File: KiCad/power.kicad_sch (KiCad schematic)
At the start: 10 parts

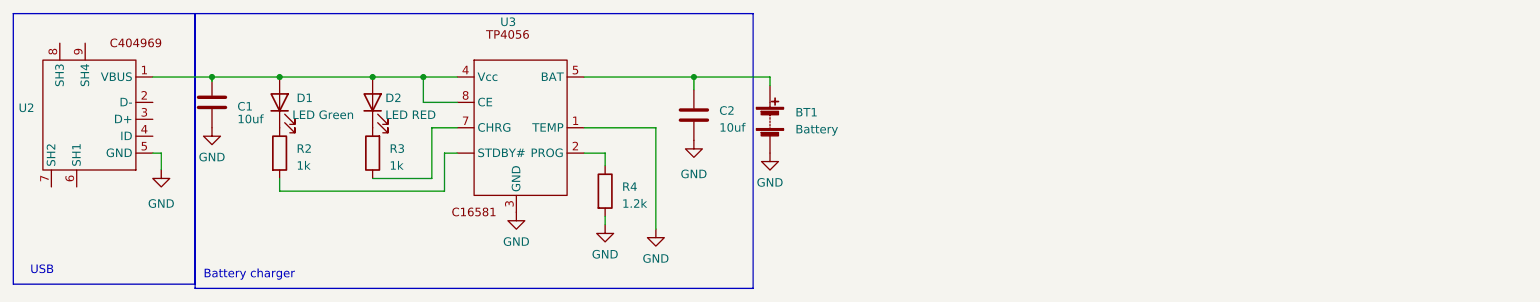
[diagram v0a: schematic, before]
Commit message: kian made som changes to the scmatices
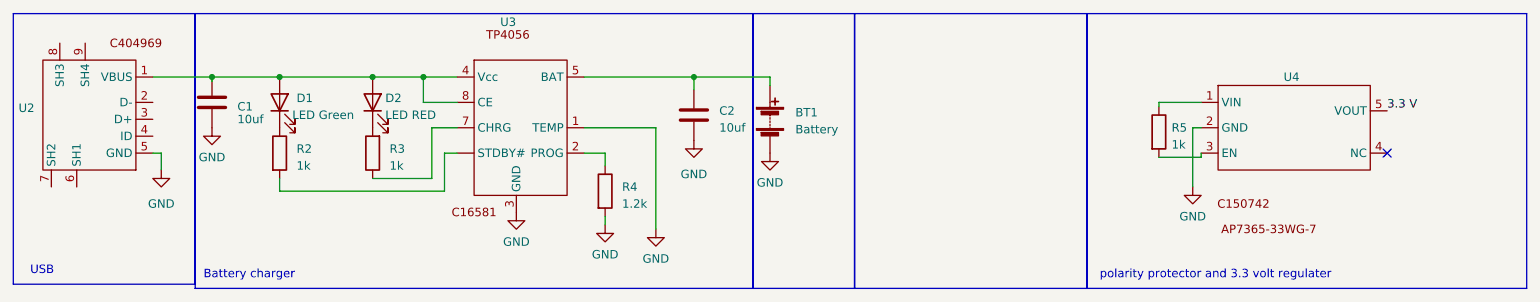
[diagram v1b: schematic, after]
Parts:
- added R5: 1k, symbol Device:R
- added U4: ~, symbol Power comonentes:C150742_(LDO/_UVLO)
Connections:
- net GND: now also U4.2 (GND)
- new net: R5.1, U4.1 (VIN)
- new net: R5.2, U4.3 (EN)
- new net 3.3 V: U4.5 (VOUT)
- no-connect marks 0 -> 1
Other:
- note added: "polarity protector and 3.3 volt regulater"
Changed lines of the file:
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@@
   (junction (at 63.5 30.48) (diameter 0) (color 0 0 0 0)
   )
+  (no_connect (at 229.87 41.91))
   (wire (pts (xy 44.45 41.91) (xy 45.72 41.91))
     (stroke (width 0) (type default))
@@
     (stroke (width 0) (type default))
   )
+  (wire (pts (xy 195.58 34.29) (xy 201.93 34.29))
+    (stroke (width 0) (type default))
+  )
   (wire (pts (xy 53.34 30.48) (xy 63.5 30.48))
     (stroke (width 0) (type default))
   )
+  (wire (pts (xy 195.58 42.545) (xy 201.93 42.545))
+    (stroke (width 0) (type default))
+  )
   (wire (pts (xy 137.16 30.48) (xy 137.16 31.75))
     (stroke (width 0) (type default))
@@
     (stroke (width 0) (type default))
   )
+  (wire (pts (xy 201.93 42.545) (xy 201.93 41.91))
+    (stroke (width 0) (type default))
+  )
   (wire (pts (xy 109.22 30.48) (xy 125.73 30.48))
     (stroke (width 0) (type default))
@@
     (stroke (width 0) (type default))
   )
+  (wire (pts (xy 195.58 34.925) (xy 195.58 34.29))
+    (stroke (width 0) (type default))
+  )
   (wire (pts (xy 85.09 34.29) (xy 85.09 30.48))
     (stroke (width 0) (type default))
@@
     (stroke (width 0) (type default))
   )
+  (wire (pts (xy 200.66 38.1) (xy 201.93 38.1))
+    (stroke (width 0) (type default))
+  )
   (wire (pts (xy 85.09 30.48) (xy 90.17 30.48))
     (stroke (width 0) (type default))
@@
     (stroke (width 0) (type default))
   )
+  (wire (pts (xy 200.66 38.1) (xy 200.66 46.99))
+    (stroke (width 0) (type default))
+  )
   (wire (pts (xy 88.265 41.91) (xy 90.17 41.91))
     (stroke (width 0) (type default))
@@
     (stroke (width 0) (type default))
   )
+  (rectangle (start 134.62 20.955) (end 149.86 62.23)
+    (stroke (width 0) (type default))
+    (fill (type none))
+  )
   (rectangle (start 50.8 20.955) (end 134.62 62.23)
     (stroke (width 0) (type default))
     (fill (type none))
   )
+  (rectangle (start 149.86 20.955) (end 184.785 62.23)
+    (stroke (width 0) (type default))
+    (fill (type none))
+  )
   (rectangle (start 23.495 20.955) (end 50.8 61.595)
+    (stroke (width 0) (type default))
+    (fill (type none))
+  )
+  (rectangle (start 184.785 20.955) (end 250.825 62.23)
     (stroke (width 0) (type default))
     (fill (type none))
@@
   )
   (text "USB" (at 26.035 60.325 0)
+    (effects (font (size 1.27 1.27)) (justify left bottom))
+  )
+  (text "polarity protector and 3.3 volt regulater" (at 186.69 60.96 0)
+    (effects (font (size 1.27 1.27)) (justify left bottom))
+  )
+  (label "3.3 V" (at 229.87 35.56 0) (fields_autoplaced)
     (effects (font (size 1.27 1.27)) (justify left bottom))
   )
@@
         )
       )
+      (project "power"
+        (path "/d9c34bc1-cf5e-42ef-a2b2-2cfbae723006"
+          (reference "D2") (unit 1)
+        )
+      )
       (project "tep work"
         (path "/dbd26d19-6d63-47f2-b172-340d78bc82ae"
@@
         )
       )
-      (project "tep work"
-        (path "/dbd26d19-6d63-47f2-b172-340d78bc82ae"
+      (project "power"
+        (path "/d9c34bc1-cf5e-42ef-a2b2-2cfbae723006"
           (reference "#PWR07") (unit 1)
         )
       )
+      (project "tep work"
+        (path "/dbd26d19-6d63-47f2-b172-340d78bc82ae"
+          (reference "#PWR07") (unit 1)
+        )
+      )
     )
   )
@@
         )
       )
+      (project "power"
+        (path "/d9c34bc1-cf5e-42ef-a2b2-2cfbae723006"
+          (reference "#PWR013") (unit 1)
+        )
+      )
       (project "tep work"
         (path "/dbd26d19-6d63-47f2-b172-340d78bc82ae"
@@
         )
       )
+      (project "power"
+        (path "/d9c34bc1-cf5e-42ef-a2b2-2cfbae723006"
+          (reference "#PWR08") (unit 1)
+        )
+      )
       (project "tep work"
         (path "/dbd26d19-6d63-47f2-b172-340d78bc82ae"
@@
       (project "EEE3088F_CKR"
         (path "/31e5d740-f3fb-4029-be8d-dfdc4f653d72/d53a003e-af2e-46c6-8ee9-c5701cef8adb"
+          (reference "#PWR011") (unit 1)
+        )
+      )
+      (project "power"
+        (path "/d9c34bc1-cf5e-42ef-a2b2-2cfbae723006"
           (reference "#PWR011") (unit 1)
         )
@@
         )
       )
+      (project "power"
+        (path "/d9c34bc1-cf5e-42ef-a2b2-2cfbae723006"
+          (reference "D1") (unit 1)
+        )
+      )
       (project "tep work"
         (path "/dbd26d19-6d63-47f2-b172-340d78bc82ae"
@@
       (project "EEE3088F_CKR"
         (path "/31e5d740-f3fb-4029-be8d-dfdc4f653d72/d53a003e-af2e-46c6-8ee9-c5701cef8adb"
+          (reference "R2") (unit 1)
+        )
+      )
+      (project "power"
+        (path "/d9c34bc1-cf5e-42ef-a2b2-2cfbae723006"
           (reference "R2") (unit 1)
         )
@@
         )
       )
+      (project "power"
+        (path "/d9c34bc1-cf5e-42ef-a2b2-2cfbae723006"
+          (reference "U2") (unit 1)
+        )
+      )
       (project "tep work"
         (path "/dbd26d19-6d63-47f2-b172-340d78bc82ae"
@@
         )
       )
-      (project "tep work"
-        (path "/dbd26d19-6d63-47f2-b172-340d78bc82ae"
+      (project "power"
+        (path "/d9c34bc1-cf5e-42ef-a2b2-2cfbae723006"
           (reference "C2") (unit 1)
         )
       )
+      (project "tep work"
+        (path "/dbd26d19-6d63-47f2-b172-340d78bc82ae"
+          (reference "C2") (unit 1)
+        )
+      )
+    )
+  )
+  (symbol (lib_id "power:GND") (at 200.66 46.99 0) (unit 1)
+    (in_bom yes) (on_board yes) (dnp no) (fields_autoplaced)
+    (property "Reference" "#PWR014" (at 200.66 53.34 0)
+      (effects (font (size 1.27 1.27)) hide)
+    )
+    (property "Value" "GND" (at 200.66 51.435 0)
+      (effects (font (size 1.27 1.27)))
+    )
+    (property "Footprint" "" (at 200.66 46.99 0)
+      (effects (font (size 1.27 1.27)) hide)
+    )
+    (property "Datasheet" "" (at 200.66 46.99 0)
+      (effects (font (size 1.27 1.27)) hide)
+    )
+    (pin "1")
+    (instances
+      (project "EEE3088F_CKR"
+        (path "/31e5d740-f3fb-4029-be8d-dfdc4f653d72/d53a003e-af2e-46c6-8ee9-c5701cef8adb"
+          (reference "#PWR014") (unit 1)
+        )
+      )
     )
   )
@@
         )
       )
+      (project "power"
+        (path "/d9c34bc1-cf5e-42ef-a2b2-2cfbae723006"
+          (reference "#PWR09") (unit 1)
+        )
+      )
       (project "tep work"
         (path "/dbd26d19-6d63-47f2-b172-340d78bc82ae"
@@
         )
       )
+      (project "power"
+        (path "/d9c34bc1-cf5e-42ef-a2b2-2cfbae723006"
+          (reference "#PWR010") (unit 1)
+        )
+      )
       (project "tep work"
         (path "/dbd26d19-6d63-47f2-b172-340d78bc82ae"
@@
         )
       )
+      (project "power"
+        (path "/d9c34bc1-cf5e-42ef-a2b2-2cfbae723006"
+          (reference "#PWR012") (unit 1)
+        )
+      )
       (project "tep work"
         (path "/dbd26d19-6d63-47f2-b172-340d78bc82ae"
@@
     )
   )
+  (symbol (lib_id "Device:R") (at 195.58 38.735 0) (unit 1)
+    (in_bom yes) (on_board yes) (dnp no) (fields_autoplaced)
+    (property "Reference" "R5" (at 197.485 38.1 0)
+      (effects (font (size 1.27 1.27)) (justify left))
+    )
+    (property "Value" "1k" (at 197.485 40.64 0)
+      (effects (font (size 1.27 1.27)) (justify left))
+    )
+    (property "Footprint" "" (at 193.802 38.735 90)
+      (effects (font (size 1.27 1.27)) hide)
+    )
+    (property "Datasheet" "~" (at 195.58 38.735 0)
+      (effects (font (size 1.27 1.27)) hide)
+    )
+    (pin "1")
+    (pin "2")
+    (instances
+      (project "EEE3088F_CKR"
+        (path "/31e5d740-f3fb-4029-be8d-dfdc4f653d72/d53a003e-af2e-46c6-8ee9-c5701cef8adb"
+          (reference "R5") (unit 1)
+        )
+      )
+    )
+  )
   (symbol (lib_id "Device:R") (at 112.395 47.625 0) (unit 1)
     (in_bom yes) (on_board yes) (dnp no) (fields_autoplaced)
@@
         )
       )
+      (project "power"
+        (path "/d9c34bc1-cf5e-42ef-a2b2-2cfbae723006"
+          (reference "R4") (unit 1)
+        )
+      )
       (project "tep work"
         (path "/dbd26d19-6d63-47f2-b172-340d78bc82ae"
@@
       (project "EEE3088F_CKR"
         (path "/31e5d740-f3fb-4029-be8d-dfdc4f653d72/d53a003e-af2e-46c6-8ee9-c5701cef8adb"
+          (reference "BT1") (unit 1)
+        )
+      )
+      (project "power"
+        (path "/d9c34bc1-cf5e-42ef-a2b2-2cfbae723006"
           (reference "BT1") (unit 1)
         )
@@
       (project "EEE3088F_CKR"
         (path "/31e5d740-f3fb-4029-be8d-dfdc4f653d72/d53a003e-af2e-46c6-8ee9-c5701cef8adb"
+          (reference "R3") (unit 1)
+        )
+      )
+      (project "power"
+        (path "/d9c34bc1-cf5e-42ef-a2b2-2cfbae723006"
           (reference "R3") (unit 1)
         )
@@
       (project "EEE3088F_CKR"
         (path "/31e5d740-f3fb-4029-be8d-dfdc4f653d72/d53a003e-af2e-46c6-8ee9-c5701cef8adb"
+          (reference "C1") (unit 1)
+        )
+      )
+      (project "power"
+        (path "/d9c34bc1-cf5e-42ef-a2b2-2cfbae723006"
           (reference "C1") (unit 1)
         )
@@
         )
       )
+      (project "power"
+        (path "/d9c34bc1-cf5e-42ef-a2b2-2cfbae723006"
+          (reference "U3") (unit 1)
+        )
+      )
       (project "tep work"
         (path "/dbd26d19-6d63-47f2-b172-340d78bc82ae"
@@
     )
   )
+  (symbol (lib_id "Power comonentes:C150742_(LDO/_UVLO)") (at 215.9 35.56 0) (unit 1)
+    (in_bom yes) (on_board yes) (dnp no) (fields_autoplaced)
+    (property "Reference" "U4" (at 215.5014 30.48 0)
+      (effects (font (size 1.27 1.27)))
+    )
+    (property "Value" "~" (at 215.9 35.56 0)
+      (effects (font (size 1.27 1.27)))
+    )
+    (property "Footprint" "" (at 215.9 35.56 0)
+      (effects (font (size 1.27 1.27)) hide)
+    )
+    (property "Datasheet" "" (at 215.9 35.56 0)
+      (effects (font (size 1.27 1.27)) hide)
+    )
+    (pin "1")
+    (pin "2")
+    (pin "3")
+    (pin "4")
+    (pin "5")
+    (instances
+      (project "EEE3088F_CKR"
+        (path "/31e5d740-f3fb-4029-be8d-dfdc4f653d72/d53a003e-af2e-46c6-8ee9-c5701cef8adb"
+          (reference "U4") (unit 1)
+        )
+      )
+    )
+  )
+  (sheet_instances
+    (path "/" (page "1"))
+  )
 )
